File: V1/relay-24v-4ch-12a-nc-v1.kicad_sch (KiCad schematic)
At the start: 24 parts, among them J1 DB141V-2.54-2P, J2 DB141V-2.54-4P, J3 DB142V-5.08-4P, J4 DB142V-5.08-4P, K1 Songle_SRD_1B, K2 Songle_SRD_1B, K3 Songle_SRD_1B, K4 Songle_SRD_1B

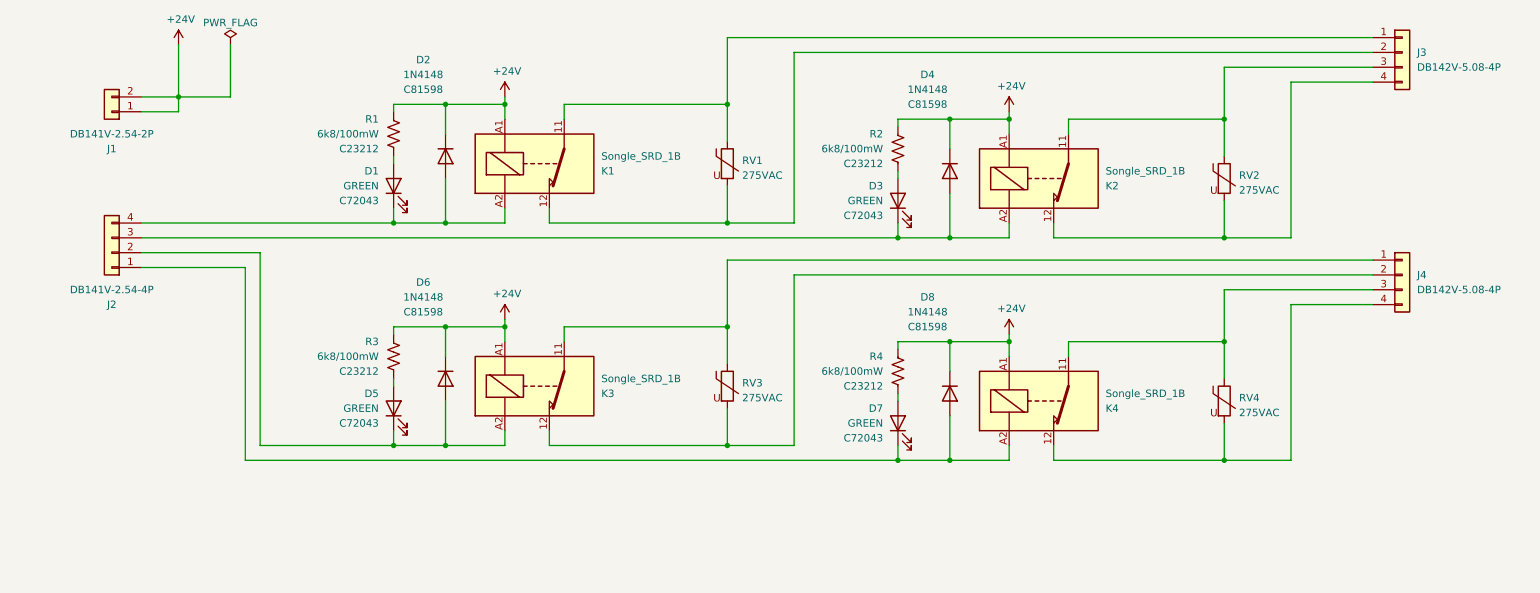
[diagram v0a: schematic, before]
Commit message: Review before fabrication
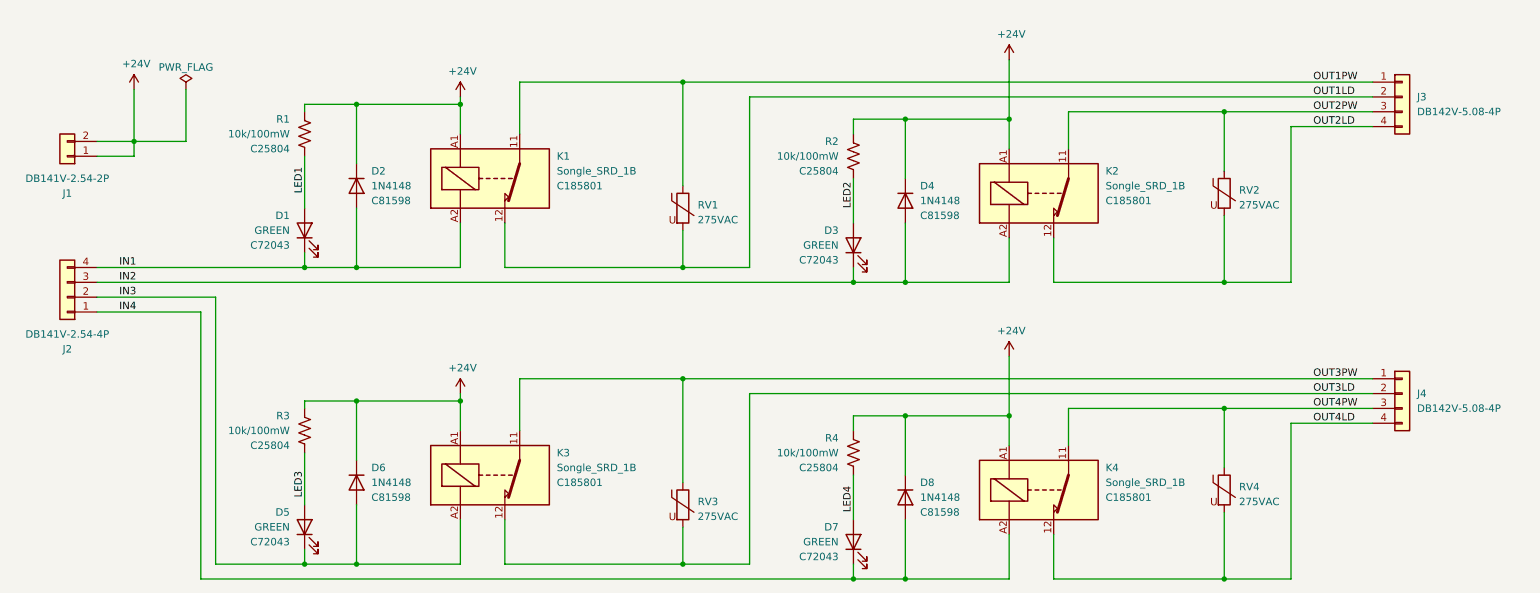
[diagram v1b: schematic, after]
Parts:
- J1, J2: JLCPCB BOM (none) -> 1; Mfr (none) -> DORABO; Vendor (none) -> JLCPCB
- R1, R2, R3, R4: value 6k8/100mW -> 10k/100mW; LCSC Part # C23212 -> C25804; Mfr Uniroyal -> UNI-ROYAL(Uniroyal Elec); Mfr PN 0603WAF6801T5E -> 0603WAF1002T5E; Vendor PN C23212 -> C25804
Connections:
- net IN4: now reaches D7.1 (K), D8.2 (A), J2.1 (Pin_1), K4.A2
- net LED4: now reaches D7.2 (A), R4.2
- net IN1: now reaches D1.1 (K), D2.2 (A), J2.4 (Pin_4), K1.A2
- net OUT3PW: now reaches J4.1 (Pin_1), K3.11, RV3.1
- net OUT3LD: now reaches J4.2 (Pin_2), K3.12, RV3.2
- net IN3: now reaches D5.1 (K), D6.2 (A), J2.2 (Pin_2), K3.A2
- net IN2: now reaches D3.1 (K), D4.2 (A), J2.3 (Pin_3), K2.A2
- net OUT2PW: now reaches J3.3 (Pin_3), K2.11, RV2.1
- net OUT2LD: now reaches J3.4 (Pin_4), K2.12, RV2.2
- net LED1: now reaches D1.2 (A), R1.2
- net LED3: now reaches D5.2 (A), R3.2
- net OUT1PW: now reaches J3.1 (Pin_1), K1.11, RV1.1
- net OUT1LD: now reaches J3.2 (Pin_2), K1.12, RV1.2
- net OUT4PW: now reaches J4.3 (Pin_3), K4.11, RV4.1
- net OUT4LD: now reaches J4.4 (Pin_4), K4.12, RV4.2
- net LED2: now reaches D3.2 (A), R2.2
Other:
- moved on the sheet: D1, D2, D3, D4, D5, D6, D7, D8, J1, J2, J3, J4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
